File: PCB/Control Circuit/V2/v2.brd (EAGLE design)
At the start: 36.2 x 35.5 mm, 6 parts, among them K1 RELAY-SPDT, Q1 60V/32A/35mΩ

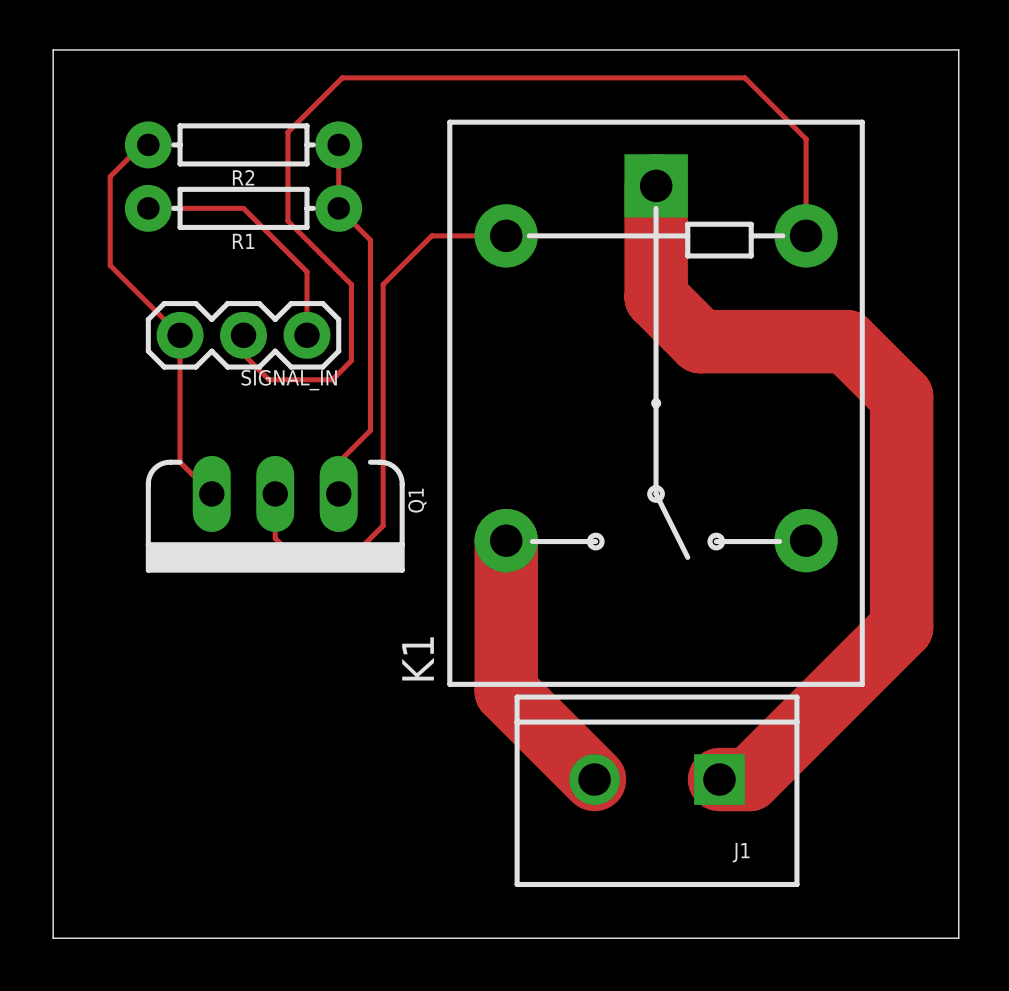
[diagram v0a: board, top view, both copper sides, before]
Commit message: Control Circuit v2
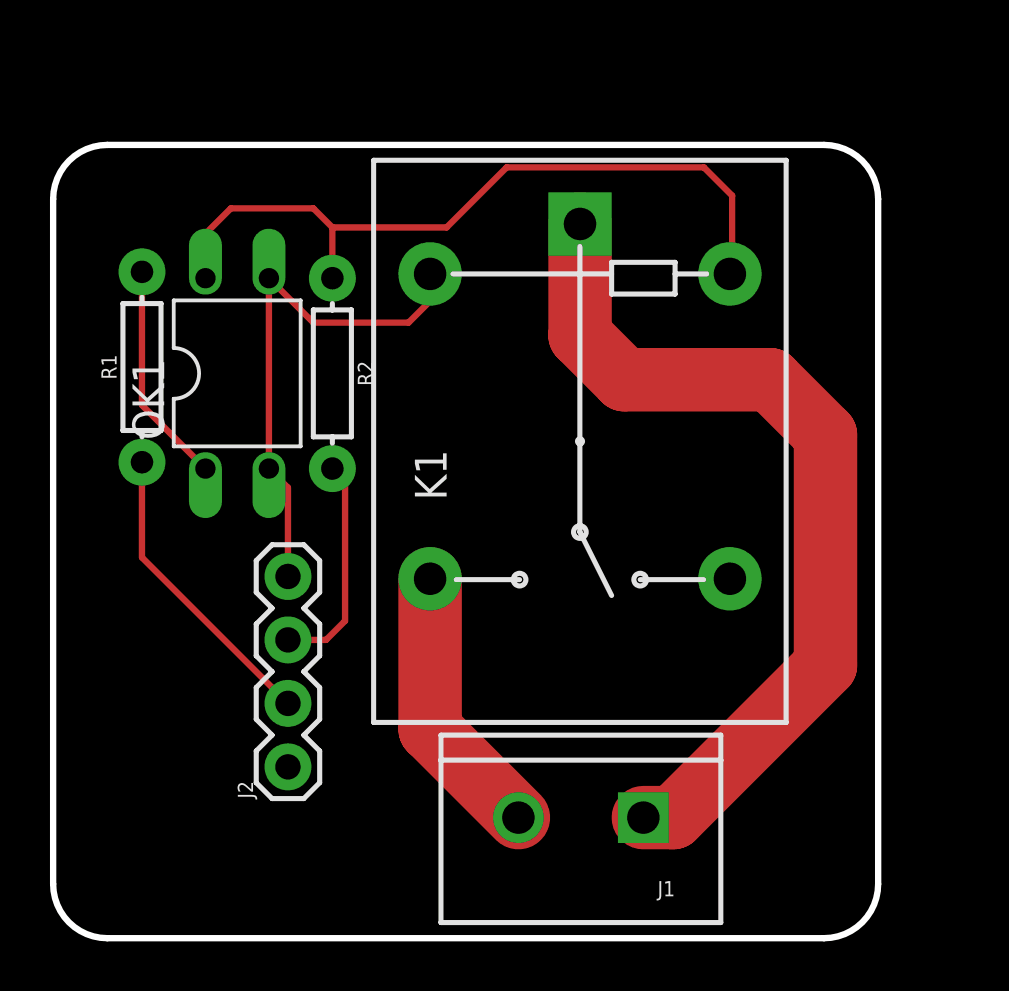
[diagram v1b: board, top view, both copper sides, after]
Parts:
- removed Q1: 60V/32A/35mΩ, SparkFun-DiscreteSemi:TO220V
- removed SIGNAL_IN: (no value), SparkFun-Connectors:1X03
- added J2: (no value), SparkFun-Connectors:1X04
- added OK1: PC817, optocoupler:DIL04
- moved R2 9.81 mm to (11.2, 22.6), turned to 270 degrees
- moved R1 7.54 mm to (3.56, 22.9), turned to 90 degrees
- moved J1 3.41 mm to (23.6, 4.83)
- moved K1 3.41 mm to (21.1, 20.1)
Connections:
- removed net N$2: K1.2, Q1.2
- new net VOUT: K1.5, OK1.4, R2.P$1
- net 5V: now also J2.3, R2.P$2; no longer K1.5, SIGNAL_IN.2
- net GND: now also J2.4, K1.2, OK1.2, OK1.3; no longer Q1.3, R2.P$2, SIGNAL_IN.3
- net N$1: now also OK1.1, R1.P$2; no longer Q1.1, R1.P$1, R2.P$1
- net TRIGGER: now also J2.2, R1.P$1; no longer R1.P$2, SIGNAL_IN.1
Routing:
- net 5V: track 42.5 -> 8.91 mm
- net VOUT: track 0.00 -> 30.3 mm
- net N$2: track 22.3 -> 0.00 mm
- net N$1: track 15.0 -> 8.93 mm
- net GND: track 16.4 -> 20.9 mm
- net TRIGGER: track 9.94 -> 12.1 mm
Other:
- board size 36.2 x 35.5 mm -> 33 x 31.8 mm
